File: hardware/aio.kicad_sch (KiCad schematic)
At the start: 9 parts, among them Q1 FCX690BTA, U1 XTR117AIDGKR, U2 ISO7021DR, U3 OPA333AIDBVR, U4 TPS78233DDCR, U5 INA219AIDCNR

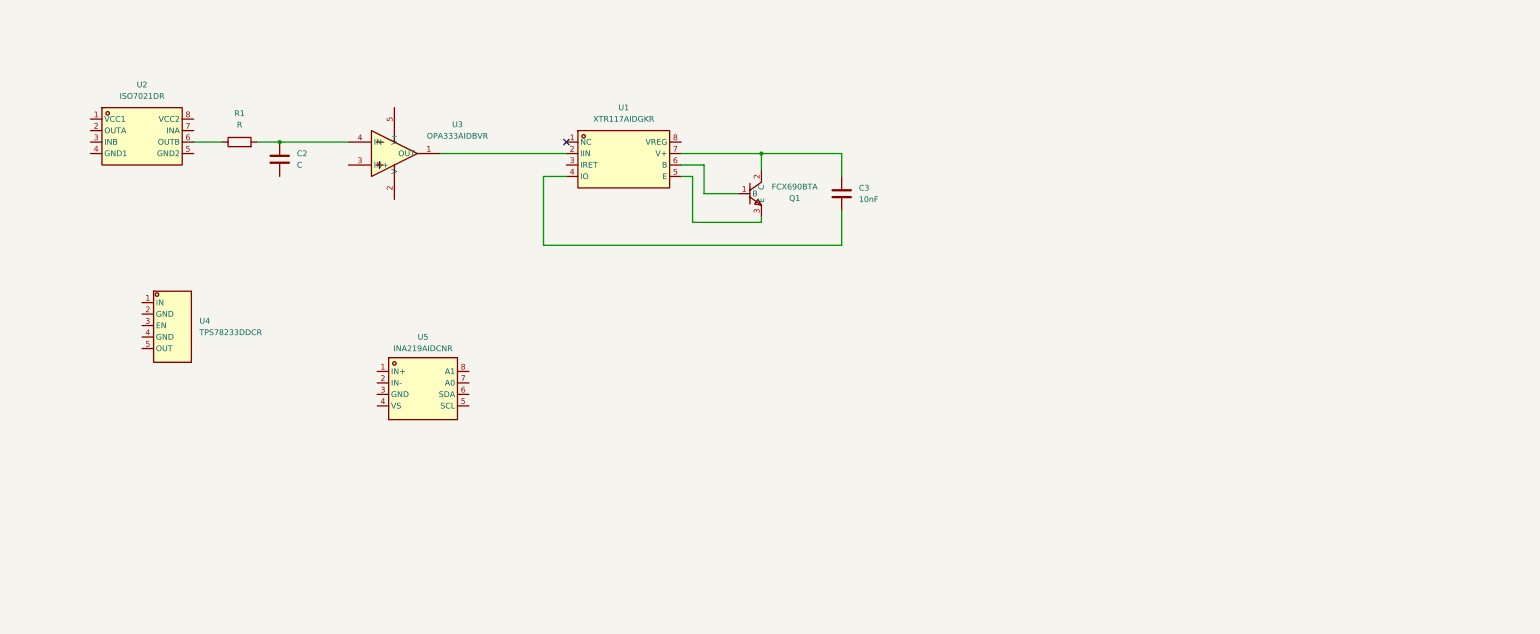
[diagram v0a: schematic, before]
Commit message: XTR117 Output
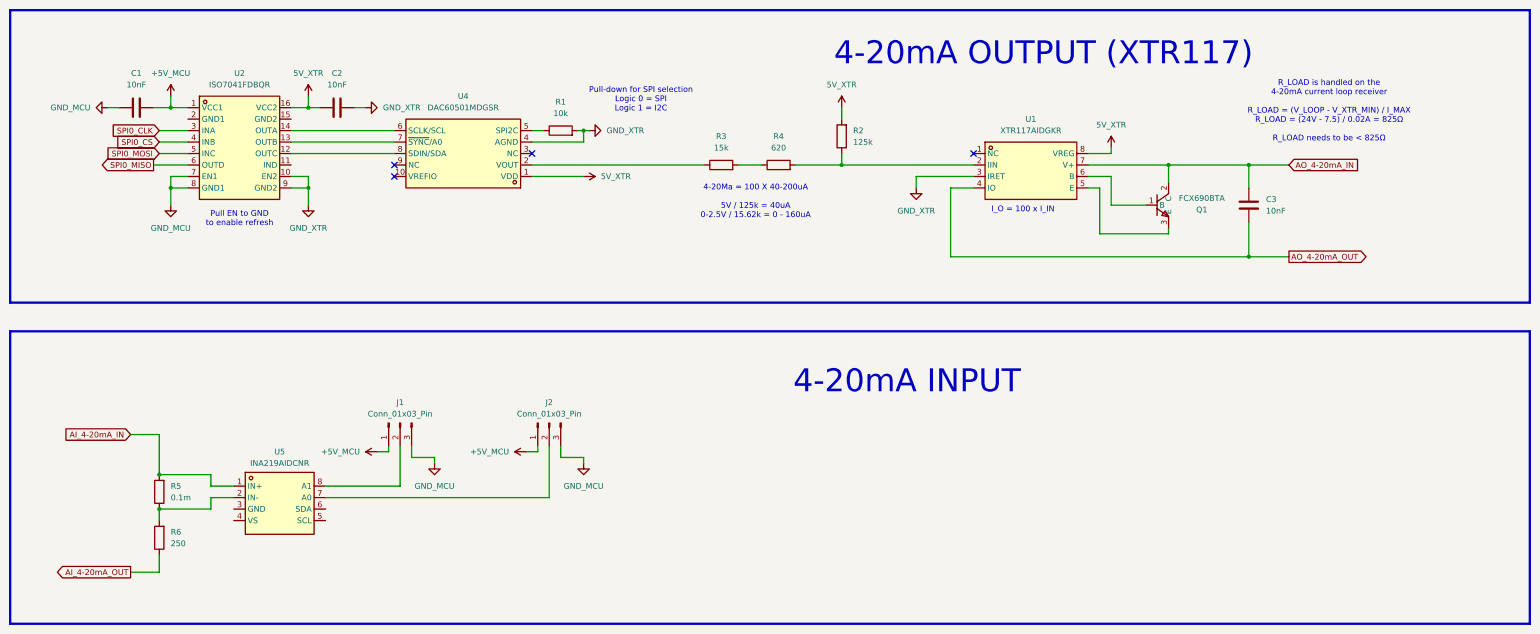
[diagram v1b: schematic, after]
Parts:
- removed U2: ISO7021DR, EasyEDA:SOIC-8_L4.9-W3.9-P1.27-LS6.0-BL, symbol EasyEDA:ISO7021DR
- removed U3: OPA333AIDBVR, EasyEDA:SOT-23-5_L3.0-W1.7-P0.95-LS2.8-BR, symbol EasyEDA:OPA333AIDBVR
- removed U4: TPS78233DDCR, EasyEDA:SOT-23-5_L3.0-W1.7-P0.95-LS2.8-BR, symbol EasyEDA:TPS78233DDCR
- added C1: 10nF, symbol Device:C
- added J1, J2: Conn_01x03_Pin, symbol Connector:Conn_01x03_Pin
- added R2: 125k, symbol Device:R
- added R3: 15k, symbol Device:R
- added R4: 620, symbol Device:R
- added R5: 0.1m, symbol Device:R
- added R6: 250, symbol Device:R
- added U2: ISO7041FDBQR, EasyEDA:SSOP-16_L4.9-W3.9-P0.64-LS6.0-BL, symbol EasyEDA:ISO7041FDBQR
- added U4: DAC60501MDGSR, EasyEDA:VSSOP-10_L3.0-W3.0-P0.50-LS4.9-BL, symbol EasyEDA:DAC60501MDGSR
- C2: value C -> 10nF
- R1: value R -> 10k
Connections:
- net at U1.2 (IIN): now also R2.1, R4.2
- net GND_XTR: now reaches U1.3 (IRET)
- net GND_XTR: now also C2.2, R1.2, U2.10 (EN2), U2.9 (GND2), U4.4 (AGND)
- net AO_4-20mA_OUT: now reaches C3.2, U1.4 (IO)
- net AO_4-20mA_IN: now reaches C3.1, Q1.2 (C), U1.7 (V+)
- net 5V_XTR: now reaches U1.8 (VREG)
- net 5V_XTR: now also C2.1, R2.2, U2.16 (VCC2), U4.1 (VDD)
- net AI_4-20mA_IN: now reaches U5.1 (IN+)
- net AI_4-20mA_IN: now also R5.2
- net at U5.2 (IN-): now also R5.1, R6.2
- net at U5.7 (A0): now also J2.2 (Pin_2)
- net at U5.8 (A1): now also J1.2 (Pin_2)
- net at R1.1: now also U4.5 (SPI2C)
- new net: R3.1, U4.2 (VOUT)
- new net: U2.14 (OUTA), U4.6 (SCLK/SCL)
- new net: U2.13 (OUTB), U4.7 (~{SYNC}/A0)
- new net: U2.12 (OUTC), U4.8 (SDIN/SDA)
- new net: R3.2, R4.1
- new net +5V_MCU: C1.2, J1.1 (Pin_1), J2.1 (Pin_1), U2.1 (VCC1)
- new net AI_4-20mA_OUT: R6.1
- new net GND_MCU: C1.1, J1.3 (Pin_3), J2.3 (Pin_3), U2.7 (EN1), U2.8 (GND1)
- new net SPI0_CLK: U2.3 (INA)
- new net SPI0_CS: U2.4 (INB)
- new net SPI0_MISO: U2.6 (OUTD)
- new net SPI0_MOSI: U2.5 (INC)
- no-connect marks 1 -> 4
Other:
- note added: "4-20Ma = 100 X 40-200uA 5V / 125k = 40uA 0-2.5V / 15.62k = 0 - 160uA"
- note added: "4-20mA INPUT"
- note added: "4-20mA OUTPUT (XTR117)"
- note added: "I_O = 100 x I_IN"
- note added: "Pull EN to GND to enable refresh"
- note added: "Pull-down for SPI selection Logic 0 = SPI Logic 1 = I2C"
- note added: "R_LOAD is handled on the 4-20mA current loop receiver R_LOAD = (V_LOOP - V_XTR_MIN) / I_MAX R_LOAD = (24V - 7.5) / 0.02A = 825Ω R_LOAD needs to be < 825Ω"
- moved on the sheet: C3, Q1, U1, U5

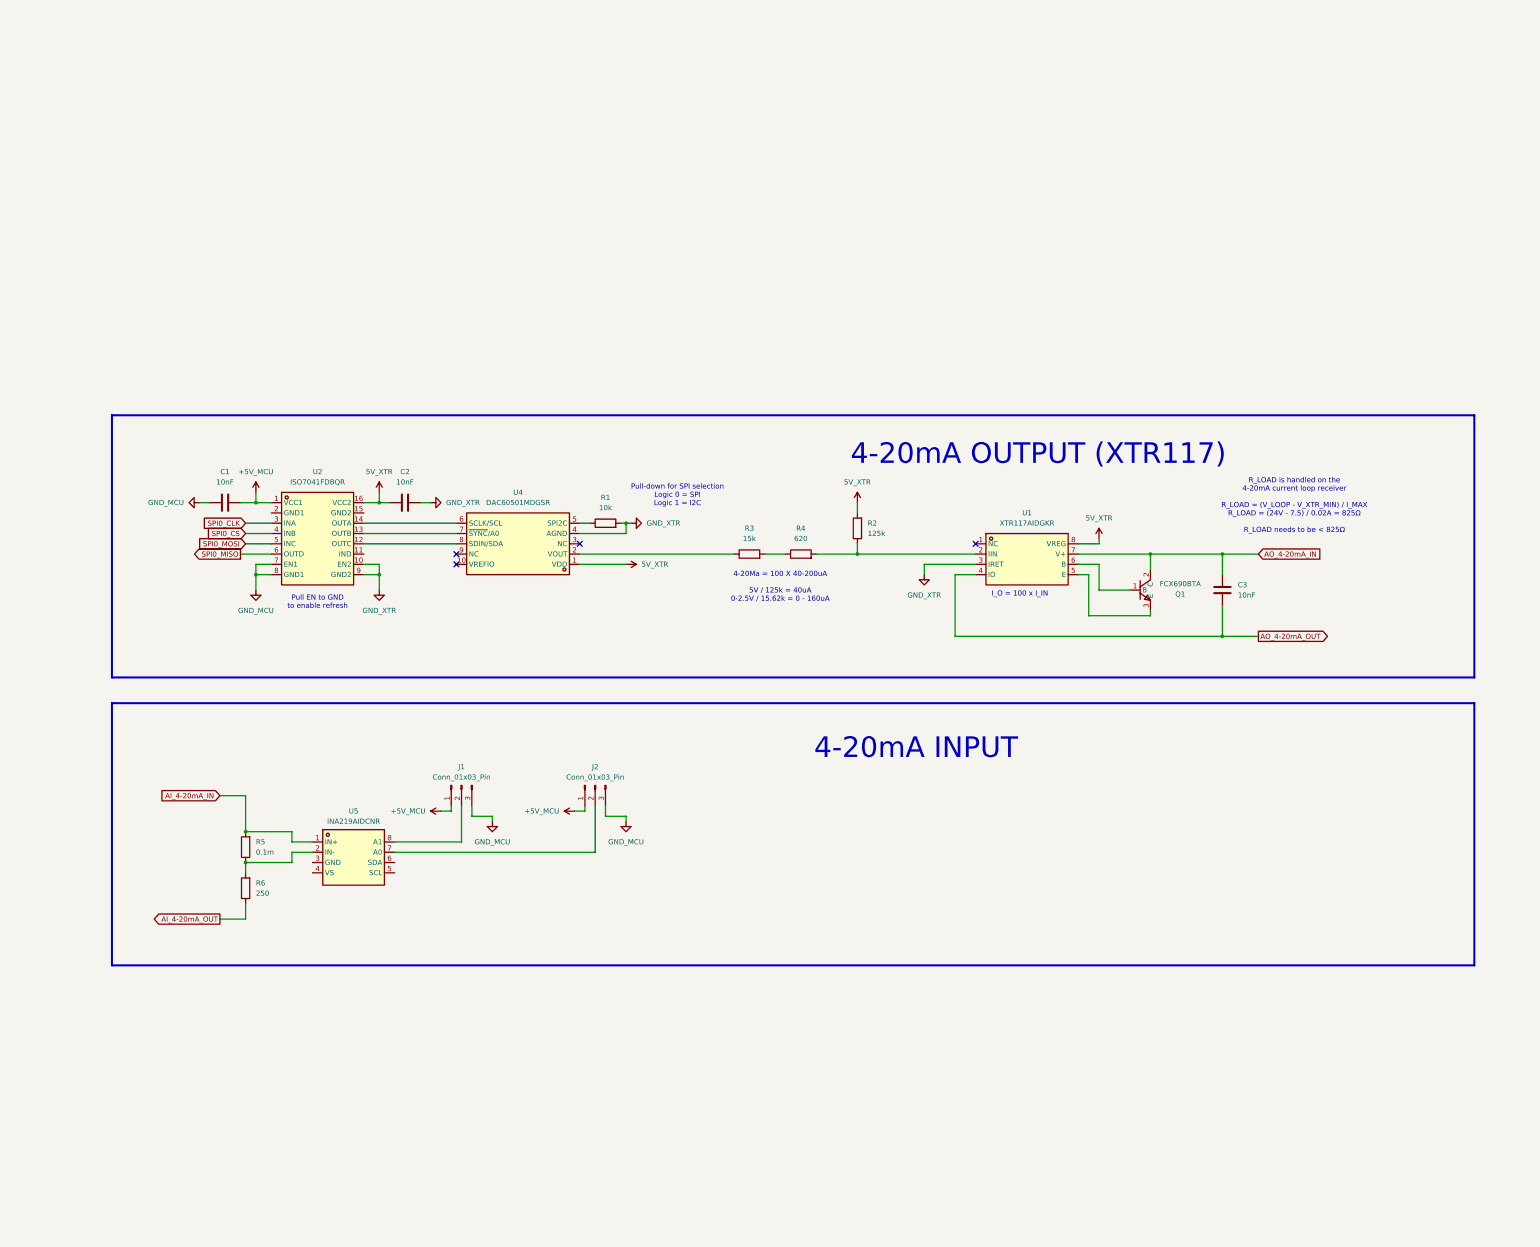
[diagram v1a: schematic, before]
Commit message: Almost everything
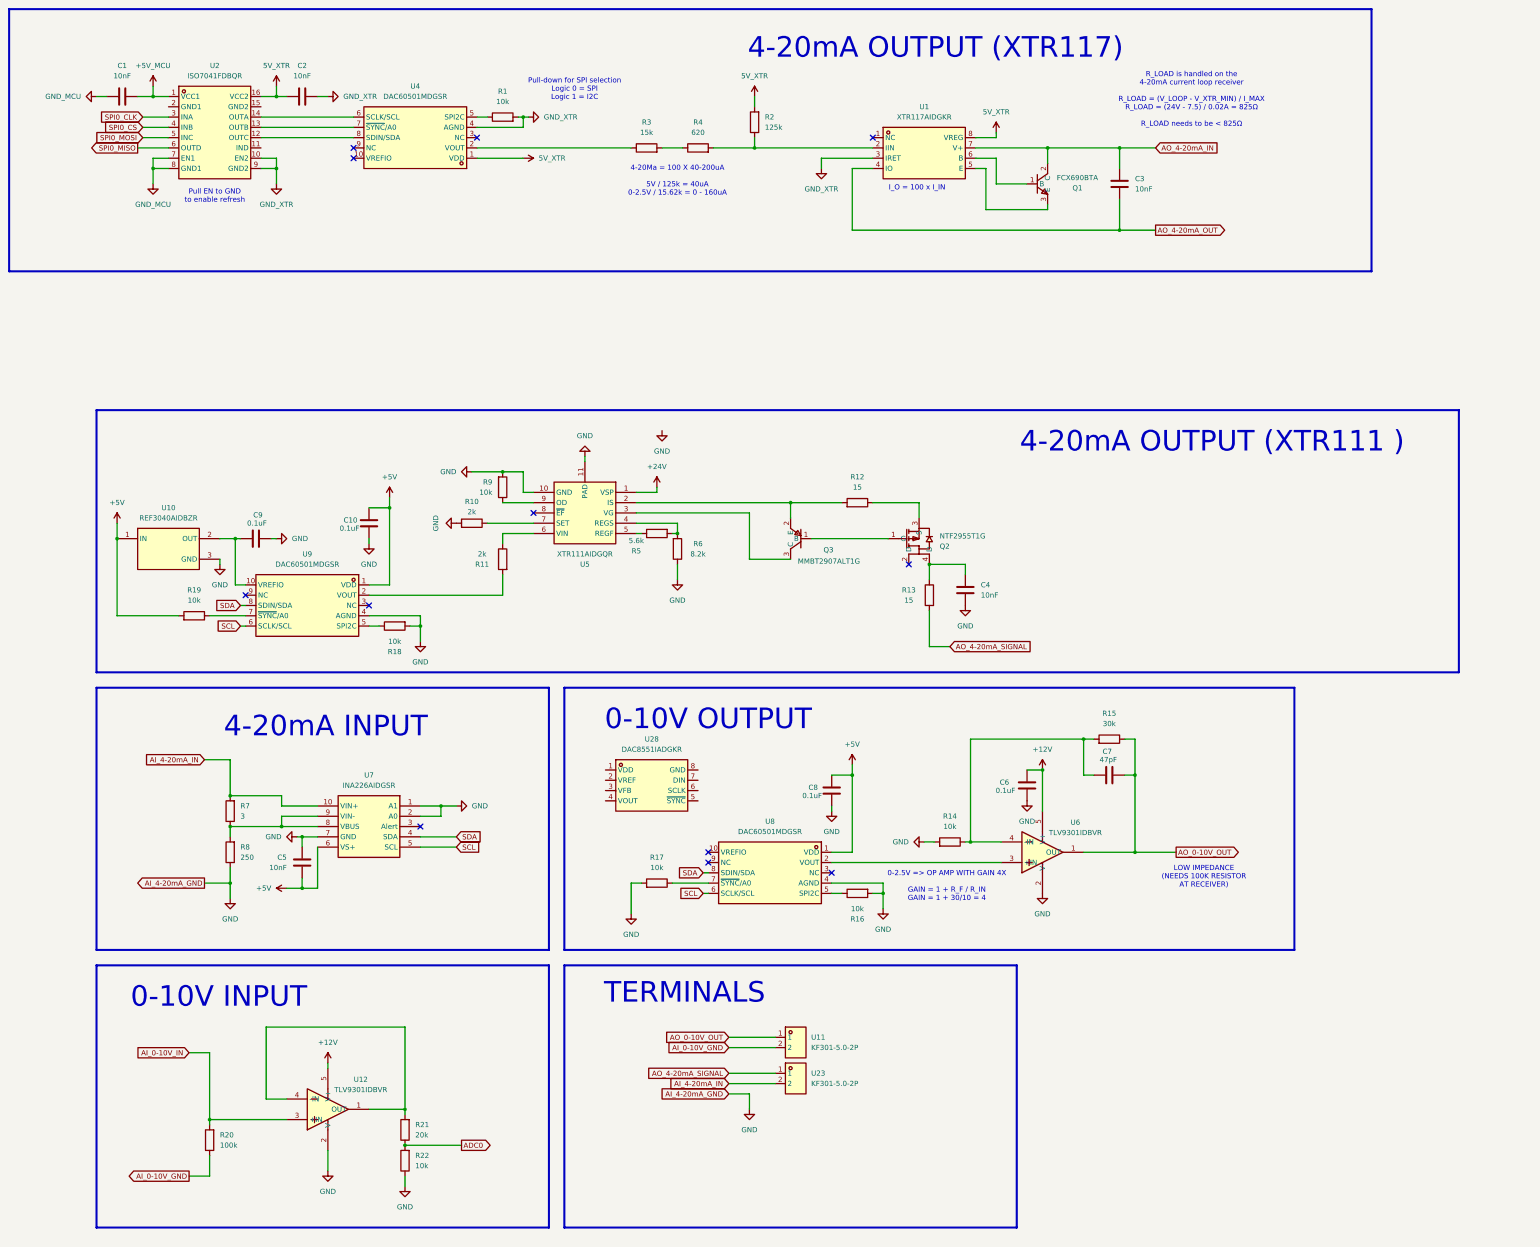
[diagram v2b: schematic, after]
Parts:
- removed J1, J2: Conn_01x03_Pin, symbol Connector:Conn_01x03_Pin
- removed U5: INA219AIDCNR, EasyEDA:SOT-23-8_L3.0-W1.7-P0.65-LS2.8-BR, symbol EasyEDA:INA219AIDCNR
- added C10, C6, C8, C9: 0.1uF, symbol Device:C
- added C4, C5: 10nF, symbol Device:C
- added C7: 47pF, symbol Device:C
- added Q2: NTF2955T1G, EasyEDA:SOT-223-4_L6.5-W3.5-P2.30-LS7.0-BR, symbol EasyEDA:NTF2955T1G
- added Q3: MMBT2907ALT1G, EasyEDA:SOT-23-3_L2.9-W1.3-P1.90-LS2.4-BR, symbol EasyEDA:MMBT2907ALT1G
- added R10, R11: 2k, symbol Device:R
- added R12, R13: 15, symbol Device:R
- added R14, R16, R17, R18, R19, R22, R9: 10k, symbol Device:R
- added R15: 30k, symbol Device:R
- added R20: 100k, symbol Device:R
- added R21: 20k, symbol Device:R
- added R7: 3, symbol Device:R
- added R8: 250, symbol Device:R
- added U10: REF3040AIDBZR, EasyEDA:SOT-23-3_L2.9-W1.6-P1.90-LS2.8-BR, symbol EasyEDA:REF3040AIDBZR
- added U11, U23: KF301-5.0-2P, EasyEDA:CONN-TH_P5.00_KF301-5.0-2P, symbol EasyEDA:KF301-5.0-2P
- added U12, U6: TLV9301IDBVR, EasyEDA:SOT-23-5_L3.0-W1.7-P0.95-LS2.8-BR, symbol EasyEDA:TLV9301IDBVR
- added U28: DAC8551IADGKR, EasyEDA:VSSOP-8_L3.0-W3.0-P0.65-LS5.0-BL, symbol EasyEDA:DAC8551IADGKR
- added U5: XTR111AIDGQR, EasyEDA:MSOP-10_L3.0-W3.0-P0.50-LS5.0-BL-EP, symbol EasyEDA:XTR111AIDGQR
- added U7: INA226AIDGSR, EasyEDA:MSOP-10_L3.0-W3.0-P0.50-LS5.0-BL, symbol EasyEDA:INA226AIDGSR
- added U8, U9: DAC60501MDGSR, EasyEDA:VSSOP-10_L3.0-W3.0-P0.50-LS4.9-BL, symbol EasyEDA:DAC60501MDGSR
- R5: value 0.1m -> 5.6k
- R6: value 250 -> 8.2k
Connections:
- net AI_4-20mA_IN: now also R7.2, U23.2, U7.10 (VIN+); no longer R5.2
- net at R5.1: now also U5.5 (REGF); no longer R6.2
- net AI_4-20mA_OUT renamed GND
- net GND: now also C10.1, C4.1, C5.2, C6.2, C8.1, C9.2, R10.2, R14.2, R16.2, R17.2, R18.2, R22.1, R8.1, R9.2, U10.3 (GND), U12.2 (V-), U5.10 (GND), U5.11 (PAD), U6.2 (V-), U7.1 (A1), U7.2 (A0), U7.7 (GND), U8.4 (AGND), U9.4 (AGND)
- new net: R10.1, U5.7 (SET)
- new net: Q2.1 (G), Q3.1 (B)
- new net: Q3.2 (E), R12.2, U5.2 (IS)
- new net: Q3.3 (C), U5.3 (VG)
- new net: R9.1, U5.9 (OD)
- new net: R7.1, R8.2, U7.8 (VBUS), U7.9 (VIN-)
- new net: R21.2, U12.1 (OUT), U12.4 (-IN)
- new net: C7.2, R14.1, R15.2, U6.4 (-IN)
- new net: R16.1, U8.5 (SPI2C)
- new net: U6.3 (+IN), U8.2 (VOUT)
- new net: R5.2, R6.2, U5.4 (REGS)
- new net: R19.1, U9.7 (~{SYNC}/A0)
- new net: R18.1, U9.5 (SPI2C)
- new net: R11.1, U5.6 (VIN)
- new net: R11.2, U9.2 (VOUT)
- new net: C4.2, Q2.4 (D), R13.1
- new net: Q2.3 (S), R12.1
- new net: R17.1, U8.7 (~{SYNC}/A0)
- new net: C9.1, U10.2 (OUT), U9.10 (VREFIO)
- new net +12V: C6.1, U12.5 (V+), U6.5 (V+)
- new net +24V: U5.1 (VSP)
- new net +5V: C10.2, C5.1, C8.2, R19.2, U10.1 (IN), U7.6 (VS+), U8.1 (VDD), U9.1 (VDD)
- new net ADC0: R21.1, R22.2
- new net AI_0-10V_GND: R20.1, U11.2
- new net AI_0-10V_IN: R20.2, U12.3 (+IN)
- new net AO_0-10V_OUT: C7.1, R15.1, U11.1, U6.1 (OUT)
- new net AO_4-20mA_SIGNAL: R13.2, U23.1
- new net SCL: U7.5 (SCL), U8.6 (SCLK/SCL), U9.6 (SCLK/SCL)
- new net SDA: U7.4 (SDA), U8.8 (SDIN/SDA), U9.8 (SDIN/SDA)
- no-connect marks 4 -> 12
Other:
- note added: "0-10V INPUT"
- note added: "0-10V OUTPUT"
- note added: "0-2.5V => OP AMP WITH GAIN 4X GAIN = 1 + R_F / R_IN GAIN = 1 + 30/10 = 4"
- note added: "4-20mA OUTPUT (XTR111 )"
- note added: "LOW IMPEDANCE (NEEDS 100K RESISTOR AT RECEIVER)"
- note added: "TERMINALS"
- moved on the sheet: C1, C2, C3, Q1, R1, R2, R3, R4, U1, U2, U4
